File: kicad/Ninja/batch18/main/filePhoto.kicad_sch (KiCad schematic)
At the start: 36 parts, among them J12 Conn_01x06_Male, J13 Conn_01x01_Male, J14 Conn_01x01_Male, J15 Conn_01x01_Male, J16 Conn_01x01_Male, J20 Conn_01x01_Male, J21 Conn_01x05_Male, J22 Conn_01x02_Male, J23 Conn_01x01_Male, J24 Conn_01x02_Male, J25 Conn_01x02_Male, J26 Conn_01x02_Male, J27 Conn_01x02_Male, U1 ADA2200ARUZ, U2 ADS1219IPWR, U3 COM1305-0.032768-EXT-T-TR, U4 LMP7717MF_NOPB

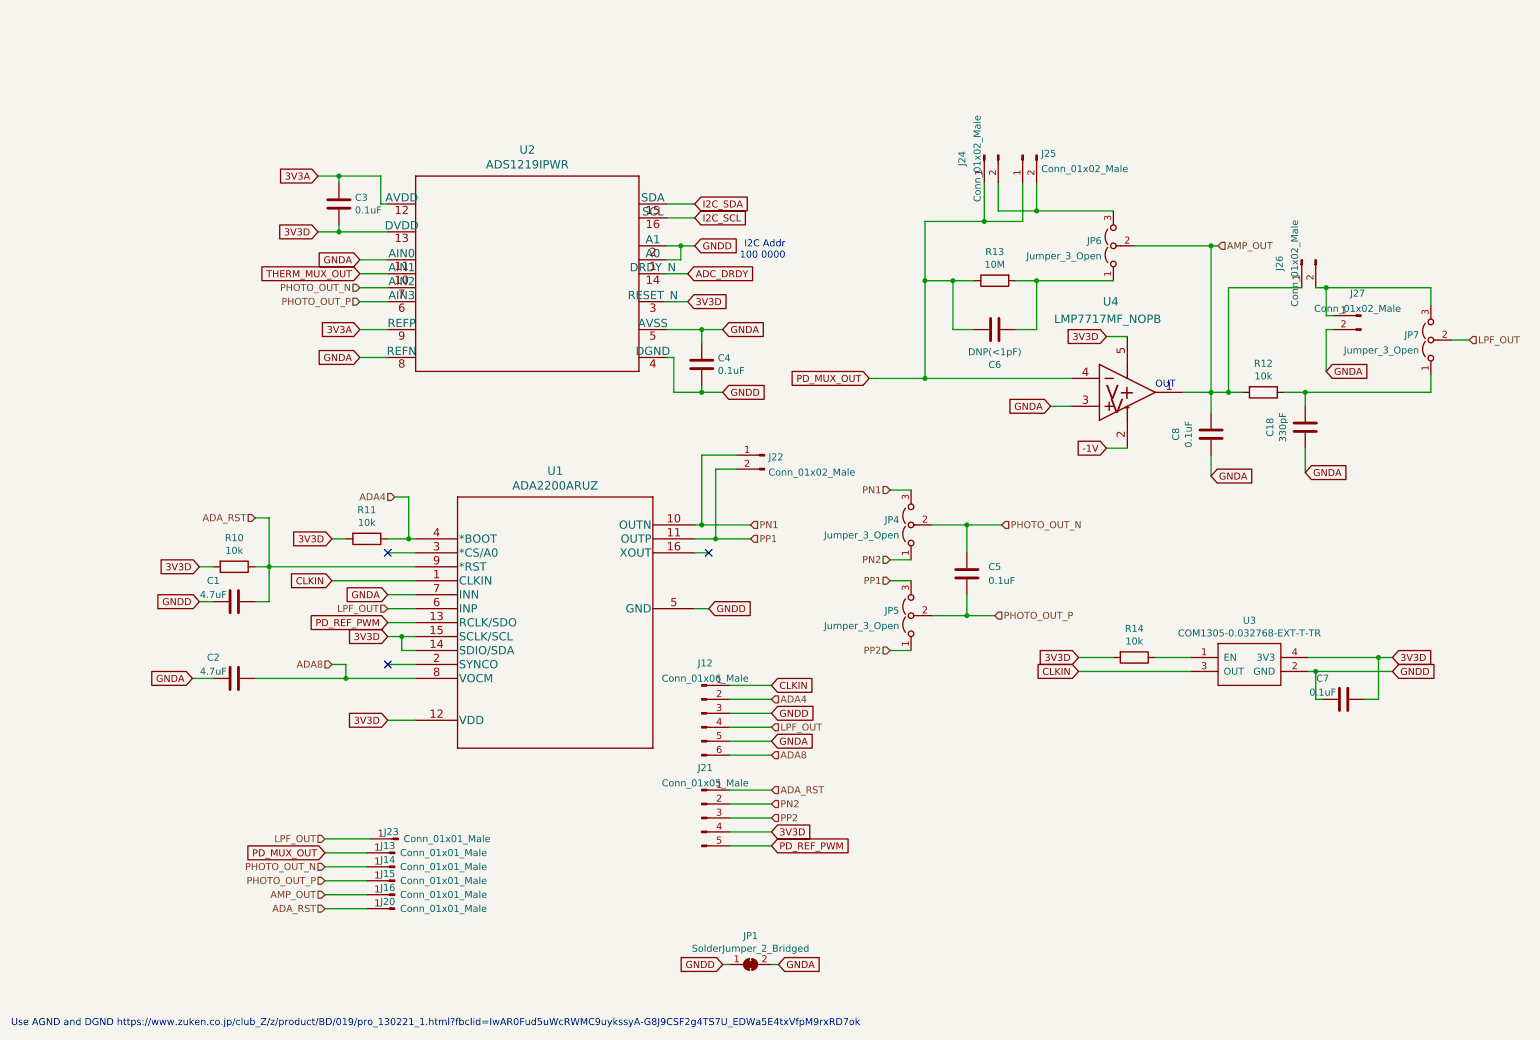
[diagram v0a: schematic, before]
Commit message: wiring batch18/main
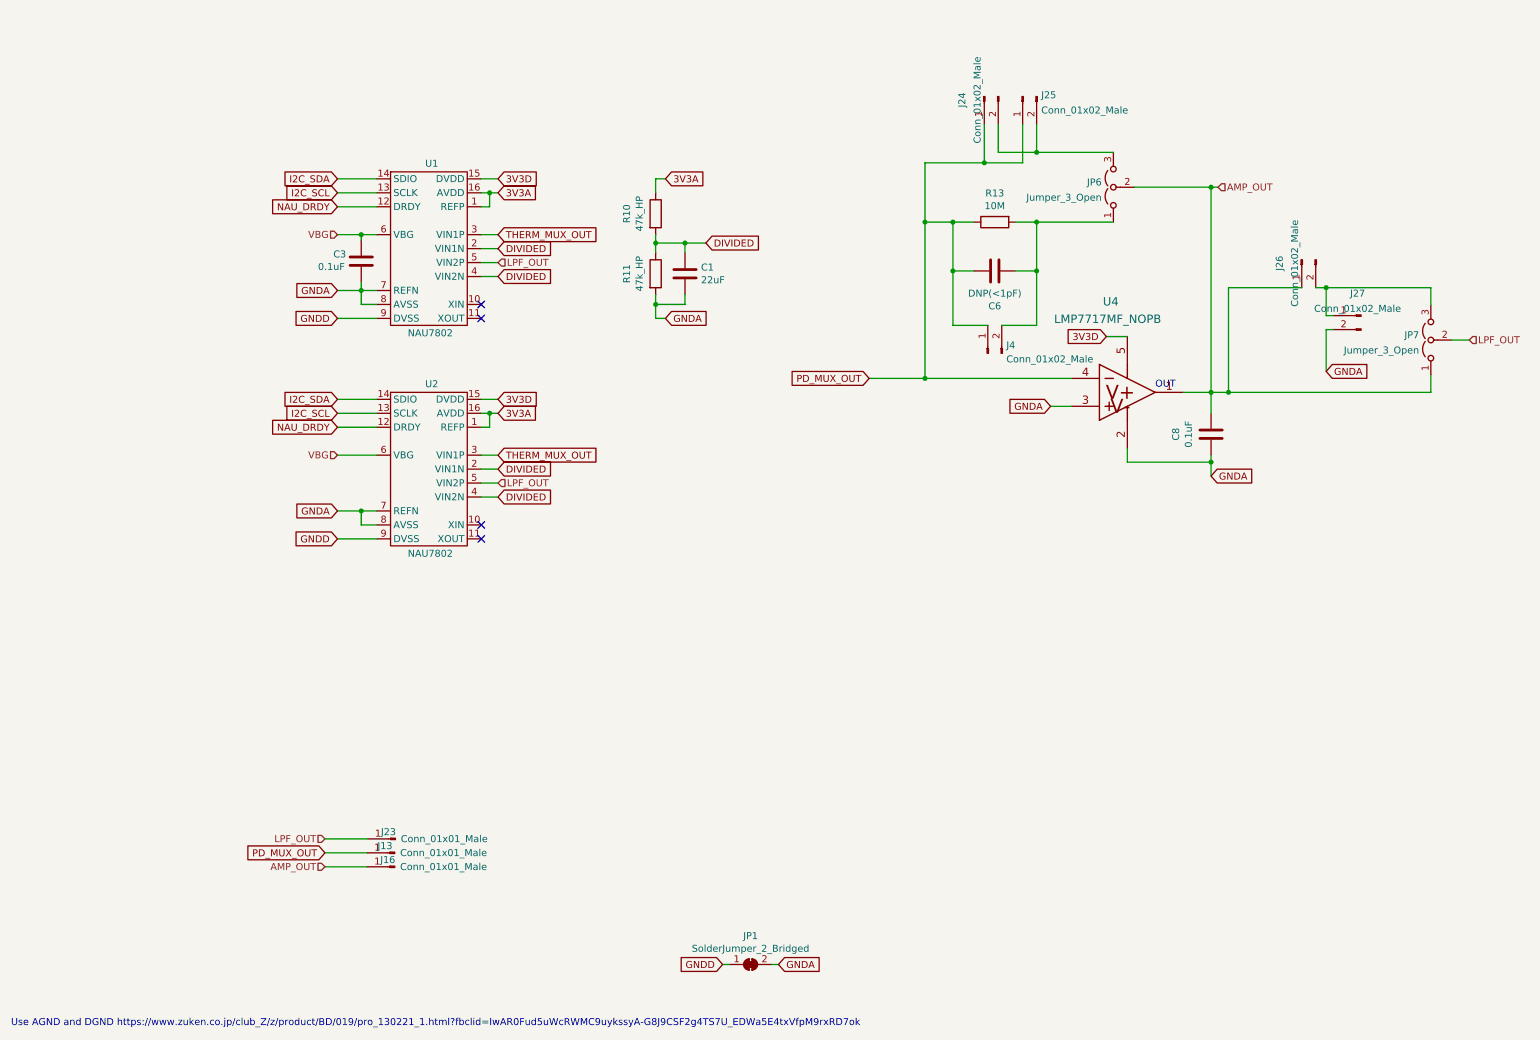
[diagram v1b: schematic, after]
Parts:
- removed C18: 330pF, Capacitor_SMD:C_0402_1005Metric, symbol Device:C
- removed C2: 4.7uF, Capacitor_SMD:C_0805_2012Metric, symbol Device:C
- removed C4, C5, C7: 0.1uF, Capacitor_SMD:C_0603_1608Metric, symbol Device:C
- removed J12: Conn_01x06_Male, Connector_PinSocket_1.27mm:PinSocket_1x06_P1.27mm_Vertical, symbol Connector:Conn_01x06_Male
- removed J14, J15: Conn_01x01_Male, Connector_PinSocket_2.54mm:PinSocket_1x01_P2.54mm_Vertical, symbol Connector:Conn_01x01_Male
- removed J20: Conn_01x01_Male, Connector_PinHeader_2.54mm:PinHeader_1x01_P2.54mm_Vertical, symbol Connector:Conn_01x01_Male
- removed J21: Conn_01x05_Male, Connector_PinSocket_1.27mm:PinSocket_1x05_P1.27mm_Vertical, symbol Connector:Conn_01x05_Male
- removed J22: Conn_01x02_Male, Connector_PinSocket_2.54mm:PinSocket_1x02_P2.54mm_Vertical, symbol Connector:Conn_01x02_Male
- removed JP4, JP5: Jumper_3_Open, Jumper:SolderJumper-3_P2.0mm_Open_TrianglePad1.0x1.5mm, symbol Jumper:Jumper_3_Open
- removed R12, R14: 10k, Resistor_SMD:R_0603_1608Metric, symbol Device:R
- removed U1: ADA2200ARUZ, Ninja-qPCR:ADA2200ARUZ, symbol Ninja-qPCR:ADA2200ARUZ
- removed U2: ADS1219IPWR, Ninja-qPCR:ADS122C04IPWR, symbol Ninja-qPCR:ADS122C04IPWR
- removed U3: COM1305-0.032768-EXT-T-TR, Ninja-qPCR:ASDK-32.768KHZ-LRT, symbol Ninja-qPCR:COM1305-0.032768-EXT-T-TR
- added J4: Conn_01x02_Male, Connector_PinHeader_2.54mm:PinHeader_1x02_P2.54mm_Vertical, symbol Connector:Conn_01x02_Male
- added U1, U2: NAU7802, symbol Ninja-qPCR:NAU7802
- C1: value 4.7uF -> 22uF; footprint Capacitor_SMD:C_0805_2012Metric -> Capacitor_SMD:C_1210_3225Metric
- R10, R11: value 10k -> 47k_HP
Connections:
- net -1V is gone; now on net GNDA: U4.2 (V-)
- net 3V3A: now also R10.1, U1.1 (REFP), U1.16 (AVDD), U2.1 (REFP), U2.16 (AVDD); no longer C3.1
- net 3V3D: now also U1.15 (DVDD), U2.15 (DVDD); no longer C3.2, R10.2, R11.2
- net AMP_OUT: now also JP7.1 (A)
- net GNDA: now also C1.1, C3.2, R11.2, U1.7 (REFN), U1.8 (AVSS), U2.7 (REFN), U2.8 (AVSS)
- net GNDD: now also U1.9 (DVSS), U2.9 (DVSS); no longer C1.2
- net I2C_SCL: now also U1.13 (SCLK), U2.13 (SCLK)
- net I2C_SDA: now also U1.14 (SDIO), U2.14 (SDIO)
- net LPF_OUT: now also U1.5 (VIN2P), U2.5 (VIN2P)
- net PD_MUX_OUT: now also J4.1 (Pin_1)
- net THERM_MUX_OUT: now also U1.3 (VIN1P), U2.3 (VIN1P)
- net at C6.1, JP6.1 (A), R13.2: now also J4.2 (Pin_2)
- net ADA4 renamed DIVIDED
- net DIVIDED: now also C1.2, R10.2, U1.2 (VIN1N), U1.4 (VIN2N), U2.2 (VIN1N), U2.4 (VIN2N)
- removed net ADA_RST: C1.1, R10.1
- new net NAU_DRDY: U1.12 (DRDY), U2.12 (DRDY)
- new net VBG: C3.1, U1.6 (VBG), U2.6 (VBG)
- no-connect marks 3 -> 4
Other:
- note removed: "I2C Addr 100 0000"
- moved on the sheet: C3, C6, J16, J23, J24, J25, JP6, R13

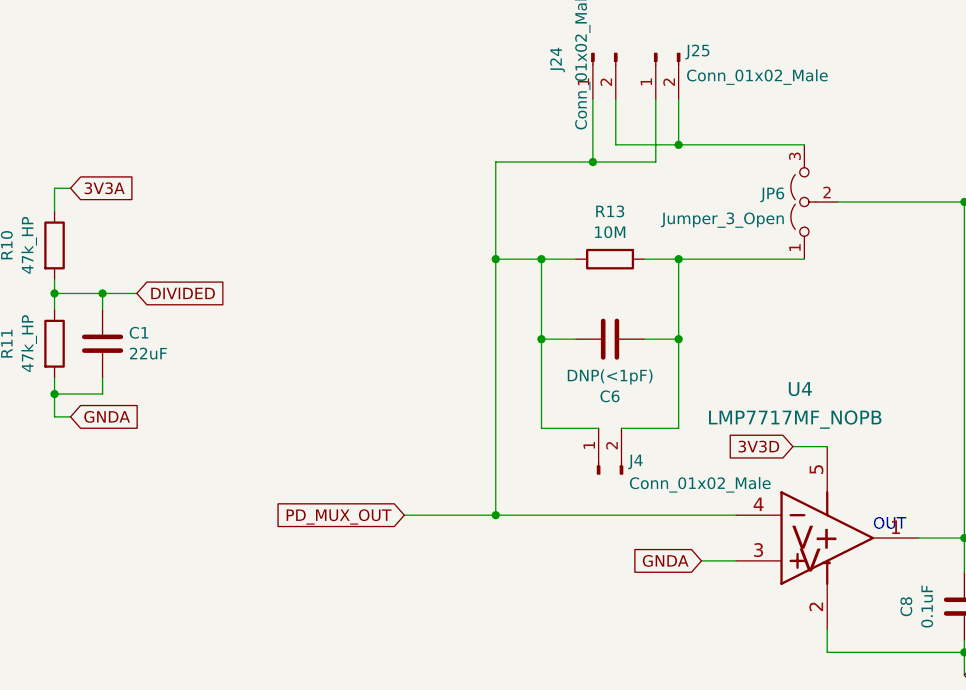
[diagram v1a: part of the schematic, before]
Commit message: apply changes from Lite
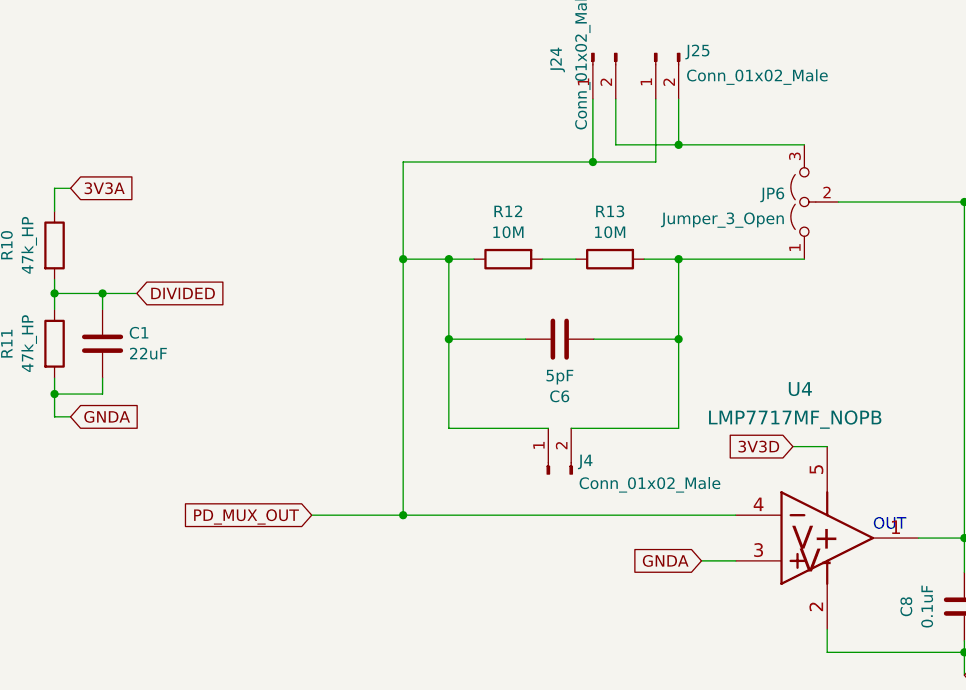
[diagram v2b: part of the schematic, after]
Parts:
- added R12: 10M, Resistor_SMD:R_0603_1608Metric, symbol Device:R
- C6: value DNP(<1pF) -> 5pF
- U1: footprint (none) -> Package_SO:SOIC-16_3.9x9.9mm_P1.27mm
- U2: footprint (none) -> Package_DIP:DIP-16_W7.62mm
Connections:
- net PD_MUX_OUT: now also R12.1; no longer R13.1
- new net: R12.2, R13.1
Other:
- moved on the sheet: C6, J4
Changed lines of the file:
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@@
   (junction (at 122.428 54.102) (diameter 0) (color 0 0 0 0)
   )
-  (junction (at 171.45 50.292) (diameter 0) (color 0 0 0 0)
+  (junction (at 161.163 50.292) (diameter 0) (color 0 0 0 0)
   )
   (junction (at 122.428 65.278) (diameter 0) (color 0 0 0 0)
@@
   (junction (at 244.475 62.23) (diameter 0) (color 0 0 0 0)
   )
-  (junction (at 176.53 50.292) (diameter 0) (color 0 0 0 0)
-  )
-  (junction (at 171.45 78.74) (diameter 0) (color 0 0 0 0)
-  )
   (junction (at 68.834 52.578) (diameter 0) (color 0 0 0 0)
   )
   (junction (at 191.77 37.592) (diameter 0) (color 0 0 0 0)
   )
+  (junction (at 166.243 59.182) (diameter 0) (color 0 0 0 0)
+  )
   (junction (at 182.245 39.497) (diameter 0) (color 0 0 0 0)
   )
@@
   (junction (at 191.77 50.292) (diameter 0) (color 0 0 0 0)
   )
-  (junction (at 176.53 59.182) (diameter 0) (color 0 0 0 0)
+  (junction (at 166.243 50.292) (diameter 0) (color 0 0 0 0)
   )
   (junction (at 127.762 54.102) (diameter 0) (color 0 0 0 0)
@@
   (junction (at 223.52 43.942) (diameter 0) (color 0 0 0 0)
   )
+  (junction (at 191.77 59.182) (diameter 0) (color 0 0 0 0)
+  )
   (junction (at 223.52 93.98) (diameter 0) (color 0 0 0 0)
   )
+  (junction (at 161.163 78.74) (diameter 0) (color 0 0 0 0)
+  )
   (junction (at 223.52 81.28) (diameter 0) (color 0 0 0 0)
-  )
-  (junction (at 191.77 59.182) (diameter 0) (color 0 0 0 0)
   )
   (no_connect (at 90.678 67.818))
@@
     (stroke (width 0) (type default) (color 0 0 0 0))
   )
-  (wire (pts (xy 185.42 69.088) (xy 191.77 69.088))
+  (wire (pts (xy 179.832 69.088) (xy 191.77 69.088))
     (stroke (width 0) (type default) (color 0 0 0 0))
   )
@@
     (stroke (width 0) (type default) (color 0 0 0 0))
   )
-  (wire (pts (xy 161.29 78.74) (xy 171.45 78.74))
+  (wire (pts (xy 151.003 78.74) (xy 161.163 78.74))
     (stroke (width 0) (type default) (color 0 0 0 0))
   )
@@
     (stroke (width 0) (type default) (color 0 0 0 0))
   )
+  (wire (pts (xy 166.243 59.182) (xy 166.243 69.088))
+    (stroke (width 0) (type default) (color 0 0 0 0))
+  )
   (wire (pts (xy 64.516 67.818) (xy 71.628 67.818))
     (stroke (width 0) (type default) (color 0 0 0 0))
@@
     (stroke (width 0) (type default) (color 0 0 0 0))
   )
-  (wire (pts (xy 180.34 59.182) (xy 176.53 59.182))
+  (wire (pts (xy 166.243 59.182) (xy 174.752 59.182))
     (stroke (width 0) (type default) (color 0 0 0 0))
   )
@@
     (stroke (width 0) (type default) (color 0 0 0 0))
   )
-  (wire (pts (xy 171.45 50.292) (xy 171.45 78.74))
-    (stroke (width 0) (type default) (color 0 0 0 0))
-  )
-  (wire (pts (xy 176.53 50.292) (xy 171.45 50.292))
+  (wire (pts (xy 161.163 50.292) (xy 161.163 78.74))
+    (stroke (width 0) (type default) (color 0 0 0 0))
+  )
+  (wire (pts (xy 166.243 50.292) (xy 161.163 50.292))
+    (stroke (width 0) (type default) (color 0 0 0 0))
+  )
+  (wire (pts (xy 166.243 50.292) (xy 169.037 50.292))
     (stroke (width 0) (type default) (color 0 0 0 0))
   )
@@
     (stroke (width 0) (type default) (color 0 0 0 0))
   )
+  (wire (pts (xy 161.163 78.74) (xy 198.12 78.74))
+    (stroke (width 0) (type default) (color 0 0 0 0))
+  )
   (wire (pts (xy 184.785 37.592) (xy 184.785 32.512))
     (stroke (width 0) (type default) (color 0 0 0 0))
@@
     (stroke (width 0) (type default) (color 0 0 0 0))
   )
-  (wire (pts (xy 176.53 59.182) (xy 176.53 50.292))
+  (wire (pts (xy 166.243 50.292) (xy 166.243 59.182))
     (stroke (width 0) (type default) (color 0 0 0 0))
   )
@@
     (stroke (width 0) (type default) (color 0 0 0 0))
   )
-  (wire (pts (xy 171.45 39.497) (xy 171.45 50.292))
+  (wire (pts (xy 161.163 39.497) (xy 161.163 50.292))
     (stroke (width 0) (type default) (color 0 0 0 0))
   )
@@
     (stroke (width 0) (type default) (color 0 0 0 0))
   )
-  (wire (pts (xy 191.77 69.088) (xy 191.77 59.182))
-    (stroke (width 0) (type default) (color 0 0 0 0))
-  )
-  (wire (pts (xy 187.96 59.182) (xy 191.77 59.182))
+  (wire (pts (xy 182.372 59.182) (xy 191.77 59.182))
     (stroke (width 0) (type default) (color 0 0 0 0))
   )
@@
     (stroke (width 0) (type default) (color 0 0 0 0))
   )
+  (wire (pts (xy 176.657 50.292) (xy 180.34 50.292))
+    (stroke (width 0) (type default) (color 0 0 0 0))
+  )
   (wire (pts (xy 204.47 71.12) (xy 208.28 71.12))
     (stroke (width 0) (type default) (color 0 0 0 0))
@@
     (stroke (width 0) (type default) (color 0 0 0 0))
   )
-  (wire (pts (xy 176.53 69.088) (xy 182.88 69.088))
+  (wire (pts (xy 166.243 69.088) (xy 177.292 69.088))
     (stroke (width 0) (type default) (color 0 0 0 0))
   )
@@
     (stroke (width 0) (type default) (color 0 0 0 0))
   )
-  (wire (pts (xy 182.245 39.497) (xy 171.45 39.497))
+  (wire (pts (xy 161.163 39.497) (xy 182.245 39.497))
     (stroke (width 0) (type default) (color 0 0 0 0))
   )
@@
     (stroke (width 0) (type default) (color 0 0 0 0))
   )
+  (wire (pts (xy 191.77 59.182) (xy 191.77 69.088))
+    (stroke (width 0) (type default) (color 0 0 0 0))
+  )
   (wire (pts (xy 62.23 165.1) (xy 69.85 165.1))
     (stroke (width 0) (type default) (color 0 0 0 0))
@@
     (stroke (width 0) (type default) (color 0 0 0 0))
   )
-  (wire (pts (xy 176.53 59.182) (xy 176.53 69.088))
-    (stroke (width 0) (type default) (color 0 0 0 0))
-  )
-  (wire (pts (xy 176.53 50.292) (xy 180.34 50.292))
-    (stroke (width 0) (type default) (color 0 0 0 0))
-  )
   (wire (pts (xy 90.678 92.71) (xy 93.726 92.71))
     (stroke (width 0) (type default) (color 0 0 0 0))
   )
   (wire (pts (xy 122.428 65.278) (xy 122.428 63.5))
-    (stroke (width 0) (type default) (color 0 0 0 0))
-  )
-  (wire (pts (xy 171.45 78.74) (xy 198.12 78.74))
     (stroke (width 0) (type default) (color 0 0 0 0))
   )
@@
     )
   )
-  (global_label "PD_MUX_OUT" (shape input) (at 161.29 78.74 180) (fields_autoplaced)
-    (effects (font (size 1.27 1.27)) (justify right))
-    (property "Intersheet References" "${INTERSHEET_REFS}" (id 0) (at 0 0 0)
+  (global_label "PD_MUX_OUT" (shape input) (at 151.003 78.74 180) (fields_autoplaced)
+    (effects (font (size 1.27 1.27)) (justify right))
+    (property "Intersheet References" "${INTERSHEET_REFS}" (id 0) (at -10.287 0 0)
       (effects (font (size 1.27 1.27)) hide)
     )
@@
     (pin "2")
   )
-  (symbol (lib_id "Device:C") (at 184.15 59.182 270) (mirror x) (unit 1)
-    (in_bom yes) (on_board yes)
-    (property "Reference" "C6" (id 0) (at 184.15 65.5828 90))
-    (property "Value" "DNP(<1pF)" (id 1) (at 184.15 63.2714 90))
-    (property "Footprint" "Capacitor_SMD:C_0603_1608Metric" (id 2) (at 180.34 58.2168 0)
-      (effects (font (size 1.27 1.27)) hide)
-    )
-    (property "Datasheet" "~" (id 3) (at 184.15 59.182 0)
+  (symbol (lib_id "Device:C") (at 178.562 59.182 270) (mirror x) (unit 1)
+    (in_bom yes) (on_board yes)
+    (property "Reference" "C6" (id 0) (at 178.562 65.5828 90))
+    (property "Value" "5pF" (id 1) (at 178.562 63.2714 90))
+    (property "Footprint" "Capacitor_SMD:C_0603_1608Metric" (id 2) (at 174.752 58.2168 0)
+      (effects (font (size 1.27 1.27)) hide)
+    )
+    (property "Datasheet" "~" (id 3) (at 178.562 59.182 0)
       (effects (font (size 1.27 1.27)) hide)
     )
@@
     (pin "1")
   )
-  (symbol (lib_id "Connector:Conn_01x02_Male") (at 182.88 74.168 90) (unit 1)
+  (symbol (lib_id "Connector:Conn_01x02_Male") (at 177.292 74.168 90) (unit 1)
     (in_bom yes) (on_board yes) (fields_autoplaced)
-    (property "Reference" "J4" (id 0) (at 186.2582 72.6983 90)
+    (property "Reference" "J4" (id 0) (at 180.6702 72.6983 90)
       (effects (font (size 1.27 1.27)) (justify right))
     )
-    (property "Value" "Conn_01x02_Male" (id 1) (at 186.2582 75.2352 90)
+    (property "Value" "Conn_01x02_Male" (id 1) (at 180.6702 75.2352 90)
       (effects (font (size 1.27 1.27)) (justify right))
     )
-    (property "Footprint" "Connector_PinHeader_2.54mm:PinHeader_1x02_P2.54mm_Vertical" (id 2) (at 182.88 74.168 0)
-      (effects (font (size 1.27 1.27)) hide)
-    )
-    (property "Datasheet" "~" (id 3) (at 182.88 74.168 0)
+    (property "Footprint" "Connector_PinHeader_2.54mm:PinHeader_1x02_P2.54mm_Vertical" (id 2) (at 177.292 74.168 0)
+      (effects (font (size 1.27 1.27)) hide)
+    )
+    (property "Datasheet" "~" (id 3) (at 177.292 74.168 0)
       (effects (font (size 1.27 1.27)) hide)
     )
@@
     (property "Reference" "U2" (id 0) (at 81.661 79.756 0))
     (property "Value" "NAU7802" (id 1) (at 81.407 110.617 0))
-    (property "Footprint" "" (id 2) (at 80.518 86.36 0)
+    (property "Footprint" "Package_DIP:DIP-16_W7.62mm" (id 2) (at 80.518 86.36 0)
       (effects (font (size 1.27 1.27)) hide)
     )
@@
     (property "Reference" "U1" (id 0) (at 81.661 39.624 0))
     (property "Value" "NAU7802" (id 1) (at 81.407 70.485 0))
-    (property "Footprint" "" (id 2) (at 80.518 46.228 0)
+    (property "Footprint" "Package_SO:SOIC-16_3.9x9.9mm_P1.27mm" (id 2) (at 80.518 46.228 0)
       (effects (font (size 1.27 1.27)) hide)
     )
@@
       (effects (font (size 1.27 1.27)) hide)
     )
+    (pin "1")
+    (pin "2")
+  )
+  (symbol (lib_id "Device:R") (at 172.847 50.292 90) (mirror x) (unit 1)
+    (in_bom yes) (on_board yes)
+    (property "Reference" "R12" (id 0) (at 172.847 45.0342 90))
+    (property "Value" "10M" (id 1) (at 172.847 47.3456 90))
+    (property "Footprint" "Resistor_SMD:R_0603_1608Metric" (id 2) (at 172.847 48.514 90)
+      (effects (font (size 1.27 1.27)) hide)
+    )
+    (property "Datasheet" "~" (id 3) (at 172.847 50.292 0)
+      (effects (font (size 1.27 1.27)) hide)
+    )
